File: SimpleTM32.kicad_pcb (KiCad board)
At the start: 2 copper layers, 41 x 36 mm, 26 parts, among them J1 USB_B_Micro, J2 Conn_01x15, J3 Conn_01x15, U1 XC6206P332MR, U2 STM32F103C8T6, Y1 8MHz

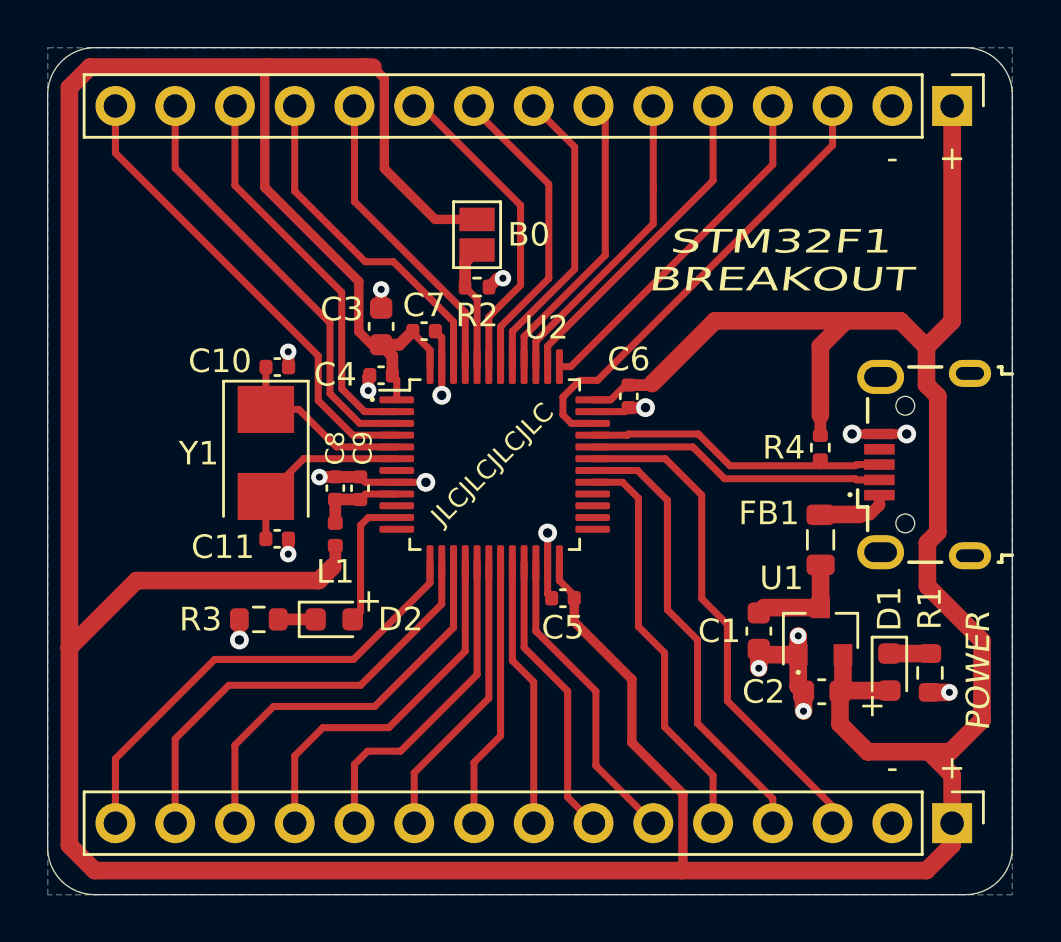
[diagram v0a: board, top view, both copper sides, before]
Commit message: on kicad 7
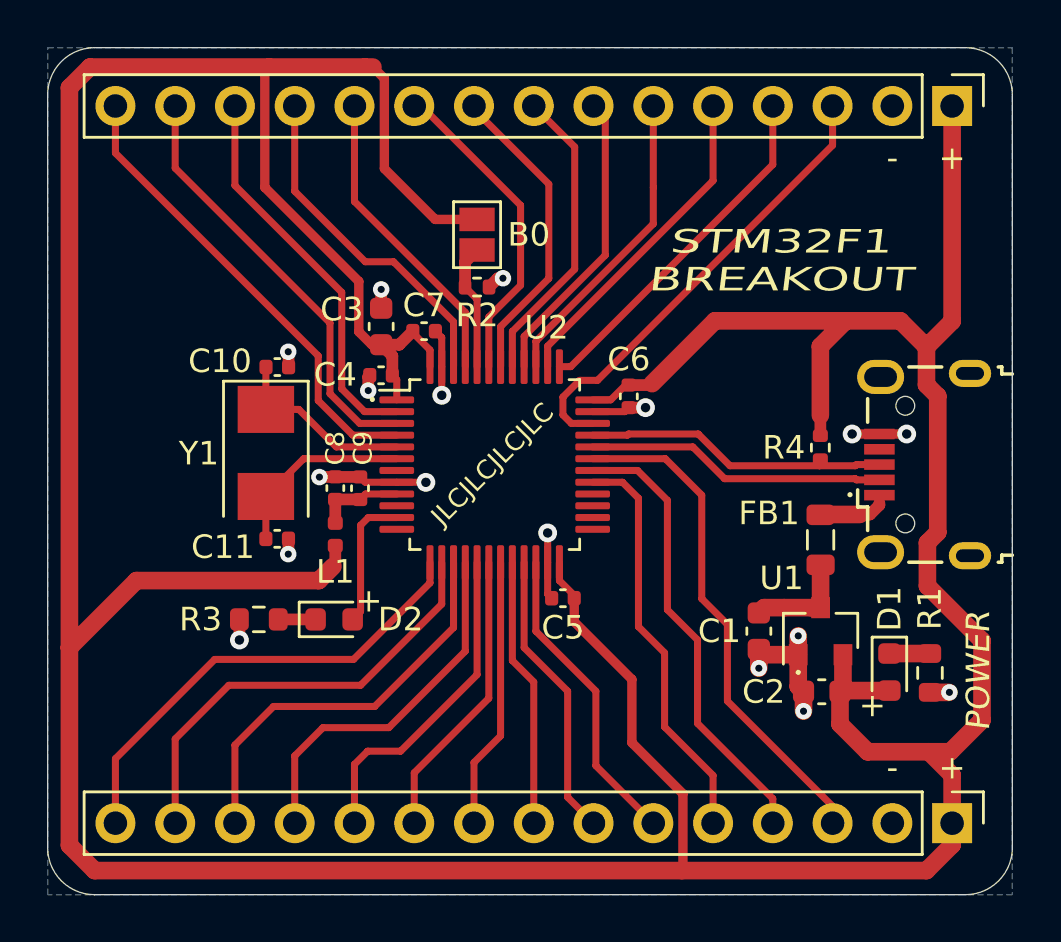
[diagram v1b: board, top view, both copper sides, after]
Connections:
- net +3V3 renamed +3.3V
- net /LED_STAT renamed Net-(D2-A)
- J1 pad 4: (no net) -> unconnected-(J1-ID-Pad4)
- U2 pad 10: (no net) -> unconnected-(U2-PA0-Pad10)
- U2 pad 12: (no net) -> unconnected-(U2-PA2-Pad12)
- U2 pad 25: (no net) -> unconnected-(U2-PB12-Pad25)
- U2 pad 26: (no net) -> unconnected-(U2-PB13-Pad26)
- U2 pad 27: (no net) -> unconnected-(U2-PB14-Pad27)
- U2 pad 28: (no net) -> unconnected-(U2-PB15-Pad28)
- U2 pad 7: (no net) -> unconnected-(U2-NRST-Pad7)
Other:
- net class Default removed
